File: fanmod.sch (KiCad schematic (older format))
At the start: 6 parts, among them J1 FAN_IN, J2 FAN_OUT, J4 COMM

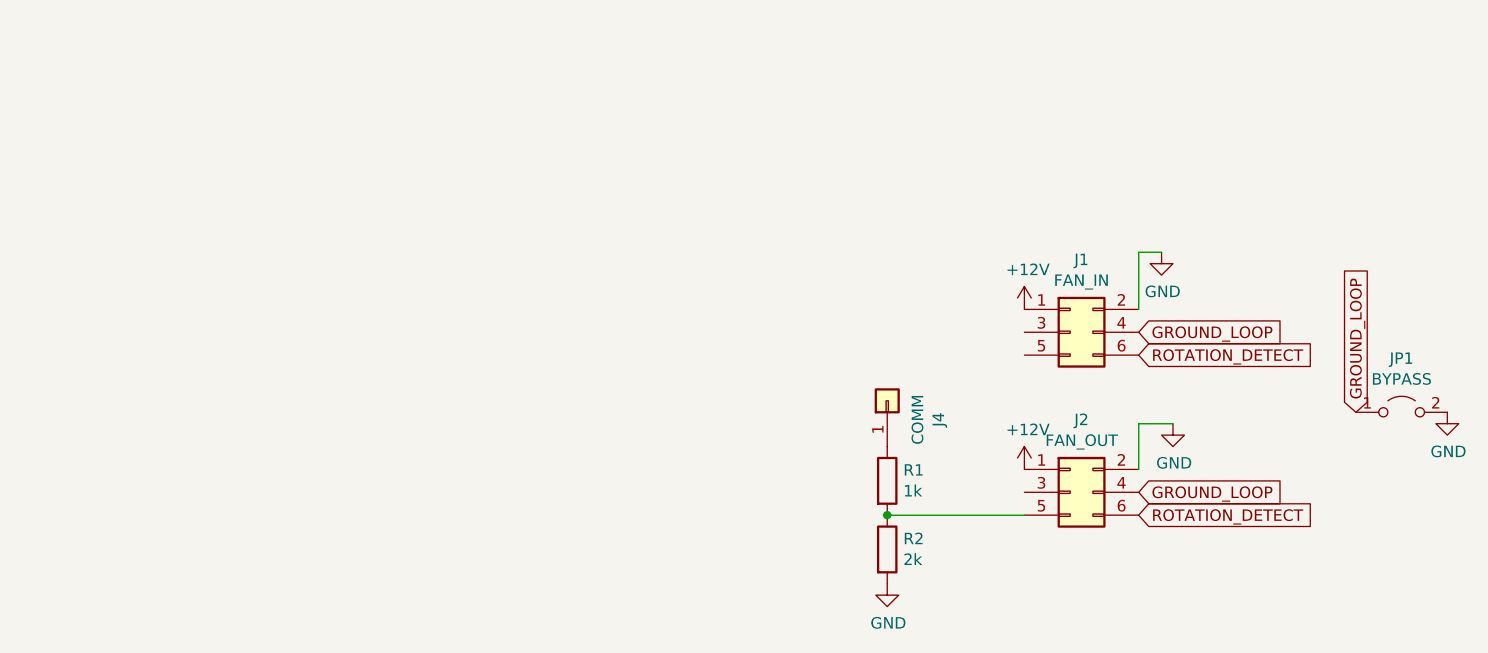
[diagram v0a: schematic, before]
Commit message: First commit
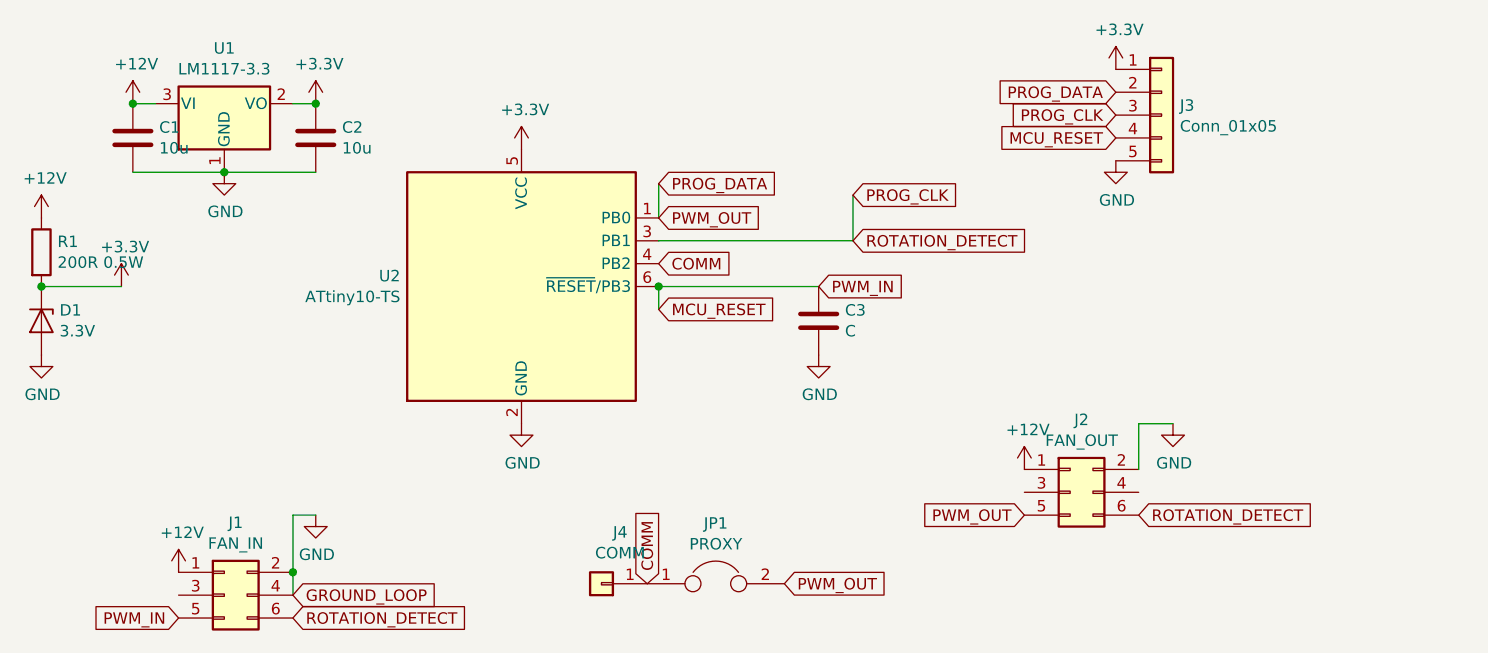
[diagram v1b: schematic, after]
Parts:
- removed JP1: BYPASS, Jumper:SolderJumper-2_P1.3mm_Open_RoundedPad1.0x1.5mm, symbol Jumper:Jumper_2_Open
- removed R2: 2k, Resistor_SMD:R_0603_1608Metric_Pad1.05x0.95mm_HandSolder, symbol Device:R
- added C1, C2: 10u, Capacitor_SMD:C_0603_1608Metric_Pad1.05x0.95mm_HandSolder, symbol Device:C
- added C3: C, Capacitor_SMD:C_0603_1608Metric_Pad1.05x0.95mm_HandSolder, symbol Device:C
- added D1: 3.3V, Diode_SMD:D_SOD-123, symbol Device:D_Zener
- added J3: Conn_01x05, Connector_PinHeader_1.27mm:PinHeader_1x05_P1.27mm_Horizontal, symbol Connector_Generic:Conn_01x05
- added JP1: PROXY, Jumper:SolderJumper-2_P1.3mm_Open_RoundedPad1.0x1.5mm, symbol Device:Jumper
- added U1: LM1117-3.3, Package_TO_SOT_SMD:SOT-223-3_TabPin2, symbol Regulator_Linear:LM1117-3.3
- added U2: ATtiny10-TS, Package_TO_SOT_SMD:SOT-23-6, symbol MCU_Microchip_ATtiny:ATtiny10-TS
- R1: value 1k -> 200R 0.5W; footprint Resistor_SMD:R_0603_1608Metric_Pad1.05x0.95mm_HandSolder -> Resistor_SMD:R_1210_3225Metric_Pad1.42x2.65mm_HandSolder
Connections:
- net +12V: now also R1.1, C1.1, U1.3 (VI)
- net GND: now also J1.4 (Pin_4), C1.2, C2.2, C3.2, D1.2 (A), J3.5 (Pin_5), U1.1 (GND), U2.2 (GND)
- net COMM: now reaches J4.1 (Pin_1)
- net COMM: now also JP1.1, U2.4 (PB2); no longer R1.1
- net +3V3: now reaches R1.2
- net +3V3: now also C2.1, D1.1 (K), J3.1 (Pin_1), U1.2 (VO), U2.5 (VCC); no longer J2.5 (Pin_5)
- net MCU_RESET: now reaches J1.5 (Pin_5)
- net MCU_RESET: now also C3.1, J3.4 (Pin_4), U2.6 (~RESET~/PB3)
- net GROUND_LOOP: no longer names the net of J2.4 (Pin_4)
- net GROUND_LOOP: no longer J1.4 (Pin_4)
- net ROTATION_DETECT renamed PROG_CLK
- net PROG_CLK: now also J3.3 (Pin_3), U2.3 (PB1)
- new net PROG_DATA: J2.5 (Pin_5), J3.2 (Pin_2), JP1.2, U2.1 (PB0)
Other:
- moved on the sheet: J1, J4
